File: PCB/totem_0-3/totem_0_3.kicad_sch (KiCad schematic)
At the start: 88 parts, among them J1 MJ-4PP-9, J2 MJ-4PP-9, U1 xiao-ble, U2 xiao-ble

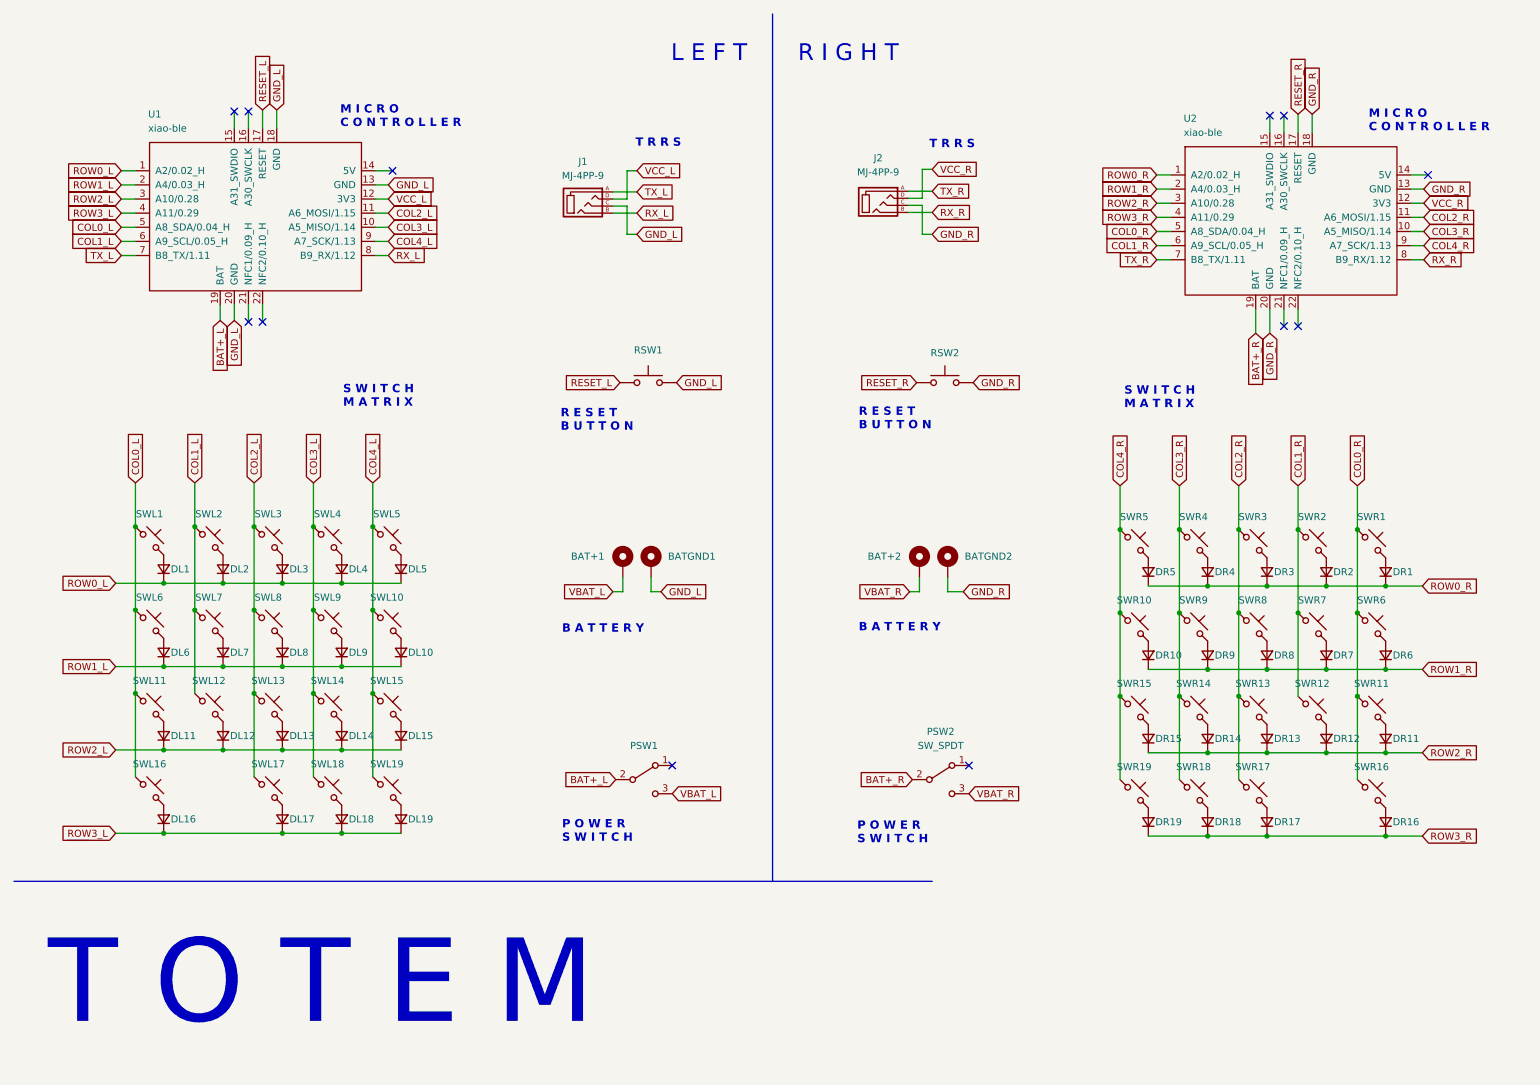
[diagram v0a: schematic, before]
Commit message: TOTEM36
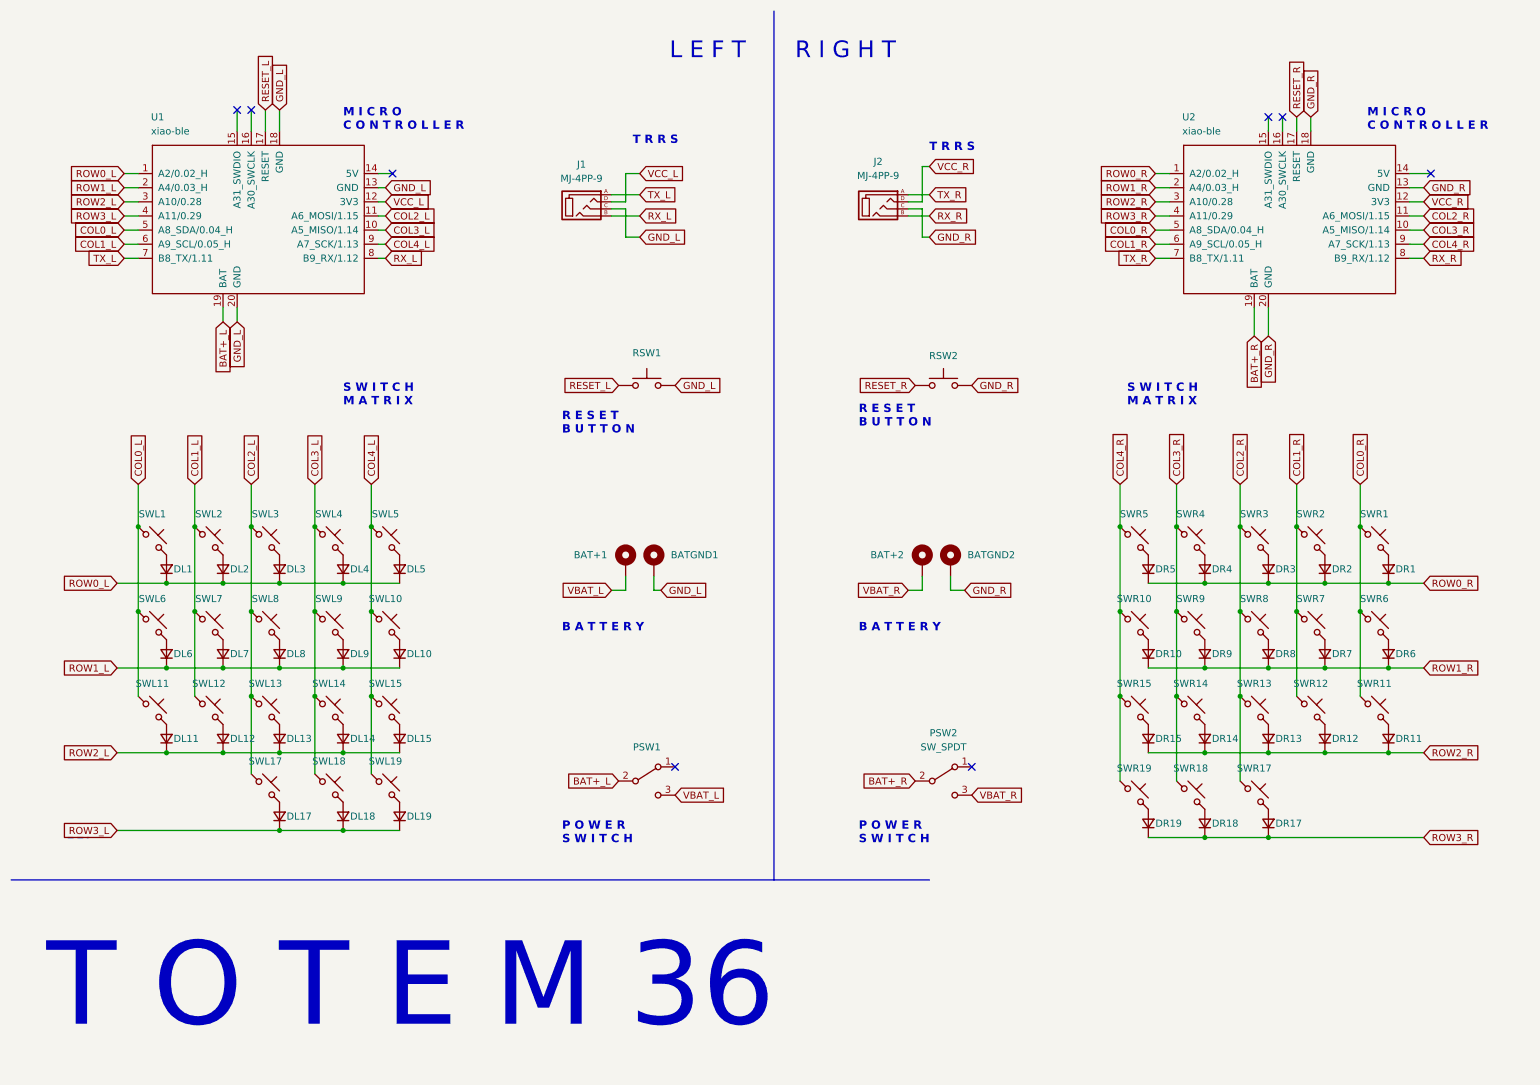
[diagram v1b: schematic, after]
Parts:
- removed DL16, DR16: D_Small, TOTEMlib:Diode_SOD123, symbol Device:D_Small
- removed SWL16, SWR16: SW_Push_45deg, TOTEMlib:Kailh_socket_PG1350_optional, symbol Switch:SW_Push_45deg
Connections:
- no-connect marks 12 -> 8
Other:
- note added: "T O T E M 36"
- note removed: "T O T E M"
- title: TOTEM split keyboard -> TOTEM36 split keyboard
- moved on the sheet: BAT+1, BAT+2, BATGND1, BATGND2, DL1, DL11, DL12, DL13, DL14, DL15, DL17, DL18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
